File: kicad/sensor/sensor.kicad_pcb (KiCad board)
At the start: 2 copper layers, 215 x 137 mm, 6 parts, among them J1 CONN, U1 150, U2 152, U3 153, U4 156, U5 155

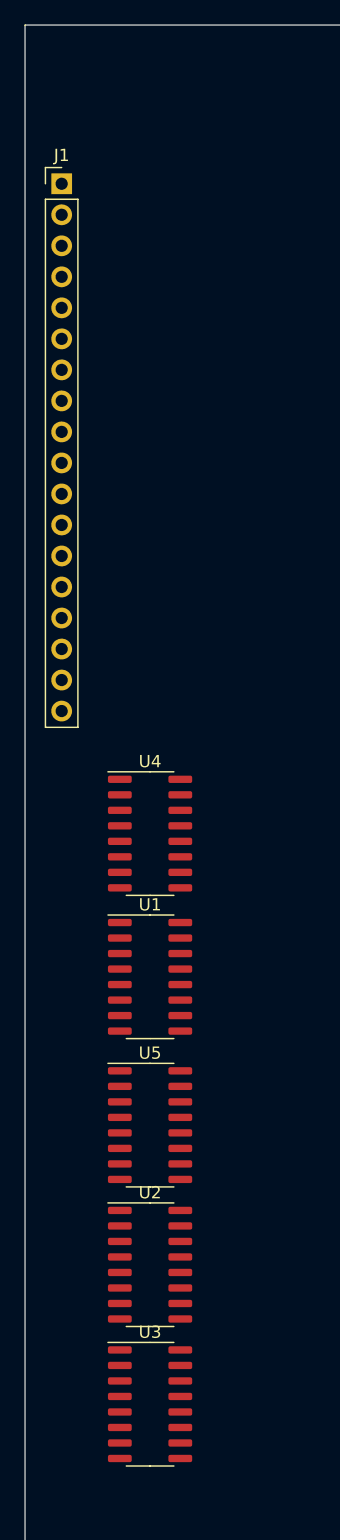
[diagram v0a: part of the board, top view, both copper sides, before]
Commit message: script update
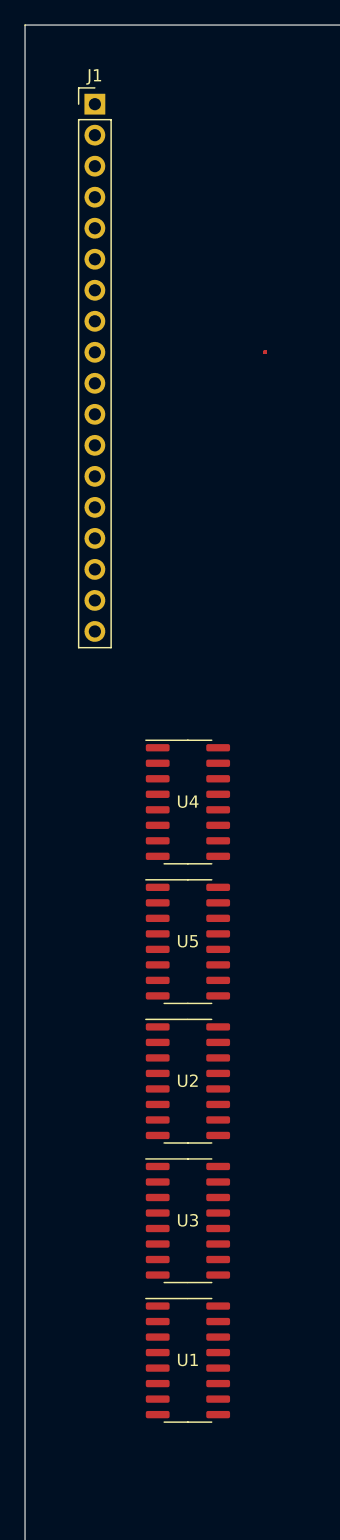
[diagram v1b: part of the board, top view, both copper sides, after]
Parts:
- added U10, U11, U12, U13, U14, U15, U16, U17, U18, U19, U20, U21, U22, U23, U24, U25, U26, U27, U28, U29, U30, U31, U32, U33, U34, U35, U36, U37, U38, U6, U7, U8, U9: jumper, jumper:jumper, F.Cu at (59.7, 50.8)
- moved U1 31.6 mm to (53.3, 133.3)
- moved U2 15.3 mm to (53.3, 110.5)
- moved U5 15.3 mm to (53.3, 99.1)
- moved U3 15.3 mm to (53.3, 121.9)
- moved J1 7.06 mm to (45.7, 30.5)
- moved U4 4.04 mm to (53.3, 87.6)
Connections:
- J1 pad 7: VCC -> VDD
- J1 pad 8: VCC -> VDD
- U1 pad 1: GND -> /X3
- U1 pad 12: GND -> /X7
- U1 pad 13: GND -> /X6
- U1 pad 14: GND -> /X5
- U1 pad 15: GND -> /X4
- U1 pad 2: GND -> /X2
- U1 pad 4: GND -> /X1
- U1 pad 5: GND -> /X0
- U2 pad 1: GND -> /X8
- U2 pad 12: GND -> /X15
- U2 pad 13: GND -> /X14
- U2 pad 14: GND -> /X13
- U2 pad 15: GND -> /X12
- U2 pad 2: GND -> /X9
- U2 pad 4: GND -> /X10
- U2 pad 5: GND -> /X11
- U3 pad 1: GND -> /X16
- U3 pad 2: GND -> /X17
- U3 pad 4: GND -> /X18
- U3 pad 5: GND -> /X19
- U4 pad 1: GND -> /Y4
- U4 pad 12: GND -> /Y0
- U4 pad 13: GND -> /Y1
- U4 pad 14: GND -> /Y2
- U4 pad 15: GND -> /Y3
- U4 pad 2: GND -> /Y5
- U4 pad 4: GND -> /Y6
- U4 pad 5: GND -> /Y7
- U5 pad 12: GND -> /Y8
- U5 pad 13: GND -> /Y9
- U5 pad 14: GND -> /Y10
- U5 pad 15: GND -> /Y11
- U5 pad 5: GND -> /Y12
- U5 pad 6: /157 -> /155

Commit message: update
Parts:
- J1, U14, U15, U16, U17, U19, U22, U23, U24, U25, U26, U27, U28, U29, U30, U31, U32, U33, U34, U35, U36, U37, U38: moved to B.Cu
- moved U23 169.4 mm to (228.3, 34.2), turned to -90 degrees
- moved U25 168.0 mm to (226.8, 34.1), turned to -90 degrees
- moved U24 153.5 mm to (212.3, 34.2), turned to -90 degrees
- moved U22 145.6 mm to (204.3, 34.2), turned to -90 degrees
- moved U3 142.1 mm to (-60.0, 36.2)
- moved U17 137.6 mm to (196.3, 34.2), turned to -90 degrees
- moved U14 129.7 mm to (188.3, 34.2), turned to -90 degrees
- moved U21 126.7 mm to (147.5, 142.2), turned to 90 degrees
- moved U5 124.3 mm to (-43.7, 21.4)
- moved U15 121.7 mm to (180.3, 34.2), turned to -90 degrees
- moved U20 121.3 mm to (139.5, 142.2), turned to 90 degrees
- moved U18 116.2 mm to (131.5, 142.2), turned to 90 degrees
- moved U16 113.8 mm to (172.3, 34.2), turned to -90 degrees
- moved U9 111.5 mm to (123.5, 142.2), turned to 90 degrees
- moved U6 107.1 mm to (115.5, 142.2), turned to 90 degrees
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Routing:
- net /Y11: track 0.00 -> 2353.6 mm, vias 0 -> 23
- net /Y3: track 0.00 -> 2345.0 mm, vias 0 -> 23
- net /Y12: track 0.00 -> 2312.4 mm, vias 0 -> 23
- net /Y1: track 0.00 -> 2308.1 mm, vias 0 -> 23
- net /Y0: track 0.00 -> 2221.6 mm, vias 0 -> 23
- net /Y4: track 0.00 -> 2221.6 mm, vias 0 -> 23
- net /Y2: track 0.00 -> 2221.6 mm, vias 0 -> 23
- net /Y7: track 0.00 -> 2221.6 mm, vias 0 -> 23
- net /Y8: track 0.00 -> 2221.6 mm, vias 0 -> 23
- net /Y5: track 0.00 -> 2221.6 mm, vias 0 -> 23
- net /Y9: track 0.00 -> 2221.6 mm, vias 0 -> 23
- net /Y6: track 0.00 -> 2221.6 mm, vias 0 -> 23
- net /Y10: track 0.00 -> 2221.6 mm, vias 0 -> 23
- net /X18: track 0.00 -> 1707.0 mm, vias 0 -> 24
- net /X19: track 0.00 -> 1678.7 mm, vias 0 -> 24
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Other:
- board text added: "fix me"

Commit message: update
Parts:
- removed U26, U27, U28, U29, U30, U31, U32, U33, U34, U35, U36, U37, U38: jumper, jumper:jumper
- moved U14 5.30 mm to (183.0, 34.1)
- moved U15 5.30 mm to (175.0, 34.1)
- moved U16 5.30 mm to (167.0, 34.1)
- moved U17 5.30 mm to (191.0, 34.1)
- moved U19 5.30 mm to (159.0, 34.1)
- moved U20 5.30 mm to (134.2, 142.1)
- moved U21 5.30 mm to (142.2, 142.1)
- moved U22 5.30 mm to (199.0, 34.1)
- moved U23 5.30 mm to (223.0, 34.1)
- moved U24 5.30 mm to (207.0, 34.1)
- moved U25 5.30 mm to (221.5, 34.0)
- moved U2 5.30 mm to (7.70, 132.9)
- moved J1 5.30 mm to (19.6, 32.3)
- moved U1 5.30 mm to (40.7, 153.9)
- moved U10 5.30 mm to (90.2, 142.1)
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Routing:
- net /Y11: track 2353.6 -> 1111.6 mm, vias 23 -> 12
- net /Y3: track 2345.0 -> 1110.7 mm, vias 23 -> 12
- net /Y12: track 2312.4 -> 1111.6 mm, vias 23 -> 12
- net /Y1: track 2308.1 -> 1110.7 mm, vias 23 -> 12
- net GND: track 108.0 -> 83.9 mm
- net /Y10: track 2221.6 -> 2222.2 mm, vias 23 -> 24
- net /Y6: track 2221.6 -> 2222.2 mm, vias 23 -> 24
- net /Y9: track 2221.6 -> 2222.2 mm, vias 23 -> 24
- net /Y5: track 2221.6 -> 2222.2 mm, vias 23 -> 24
- net /Y8: track 2221.6 -> 2222.2 mm, vias 23 -> 24
- net /Y7: track 2221.6 -> 2222.2 mm, vias 23 -> 24
- net /Y2: track 2221.6 -> 2222.2 mm, vias 23 -> 24
- net /Y4: track 2221.6 -> 2222.2 mm, vias 23 -> 24
- net /Y0: track 2221.6 -> 2222.2 mm, vias 23 -> 24
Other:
- board text removed: "fix me"

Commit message: tmp
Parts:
- moved U3 137.7 mm to (40.7, 124.0)
- moved U5 125.5 mm to (40.7, 109.0)
- moved U2 51.0 mm to (40.7, 94.0)
- moved U25 17.0 mm to (206.5, 42.0)
- moved U14 11.6 mm to (174.5, 42.0)
- moved U15 11.6 mm to (166.5, 42.0)
- moved U16 11.6 mm to (158.5, 42.0)
- moved U17 11.6 mm to (182.5, 42.0)
- moved U19 11.6 mm to (150.5, 42.0)
- moved U22 11.6 mm to (190.5, 42.0)
- moved U24 11.6 mm to (198.5, 42.0)
- moved U23 11.3 mm to (214.9, 42.0)
- moved U4 0.10 mm to (40.7, 142.0)
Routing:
- net /Y11: track 1111.6 -> 2466.3 mm, vias 12 -> 13
- net /Y3: track 1110.7 -> 2419.3 mm, vias 12 -> 24
- net /Y12: track 1111.6 -> 2272.5 mm
- net /Y1: track 1110.7 -> 2234.6 mm, vias 12 -> 24
- net /X3: track 954.8 -> 1720.2 mm, vias 20 -> 14
- net /X1: track 880.5 -> 1539.3 mm, vias 20 -> 14
- net /X19: track 1678.7 -> 1477.8 mm, vias 24 -> 14
- net /X18: track 1707.0 -> 1901.7 mm, vias 24 -> 14
- net GND: track 83.9 -> 254.7 mm
- net /Y10: track 2222.2 -> 2366.6 mm
- net /X17: track 1562.2 -> 1697.5 mm, vias 24 -> 26
- net /X16: track 1562.2 -> 1694.9 mm, vias 24 -> 26
- net /Y0: track 2222.2 -> 2344.4 mm
- net /X15: track 1562.2 -> 1682.2 mm, vias 24 -> 26
- net /X14: track 1562.2 -> 1673.4 mm, vias 24 -> 26
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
